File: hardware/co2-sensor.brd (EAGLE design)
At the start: 40 x 44 mm, 21 parts, among them IC1 LM1117IMPX-3.3, J1 MH-Z19, U1 esp12e, U2 dht22, U3 BMP280

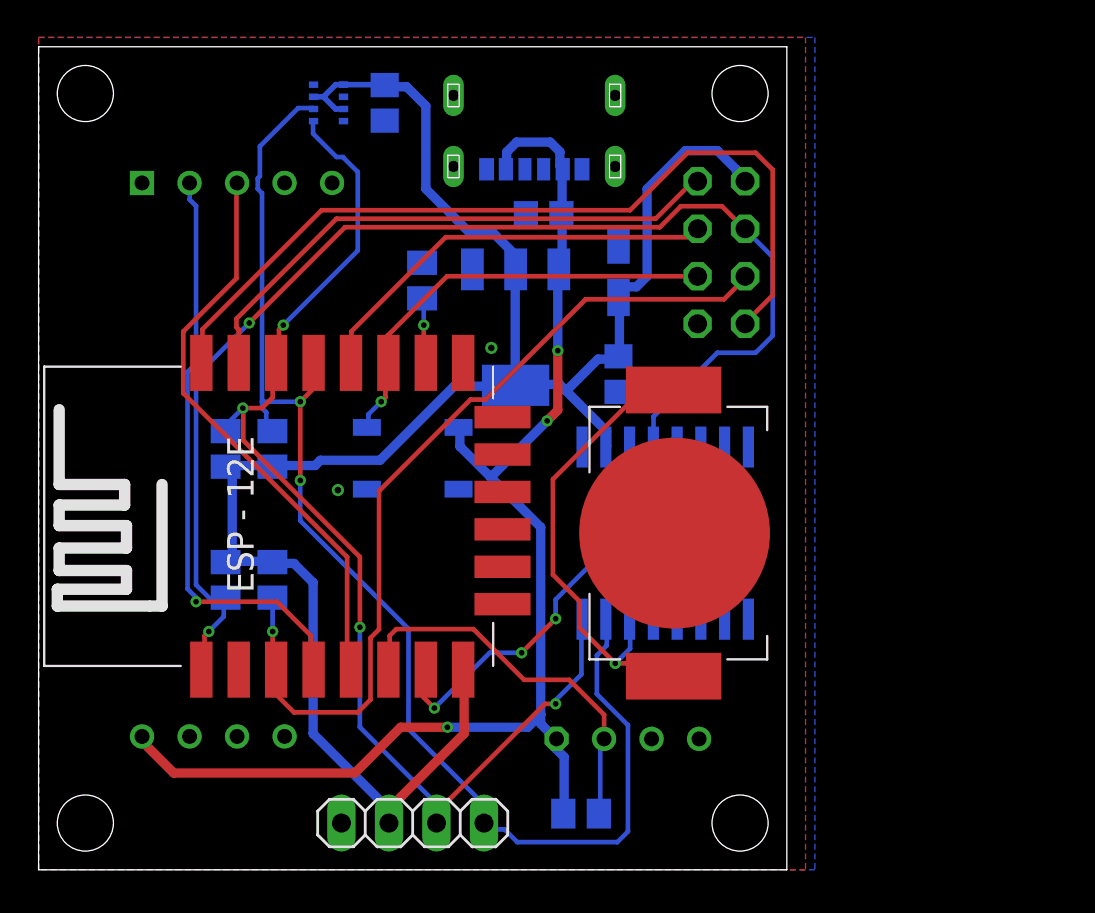
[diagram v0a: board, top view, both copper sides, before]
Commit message: .
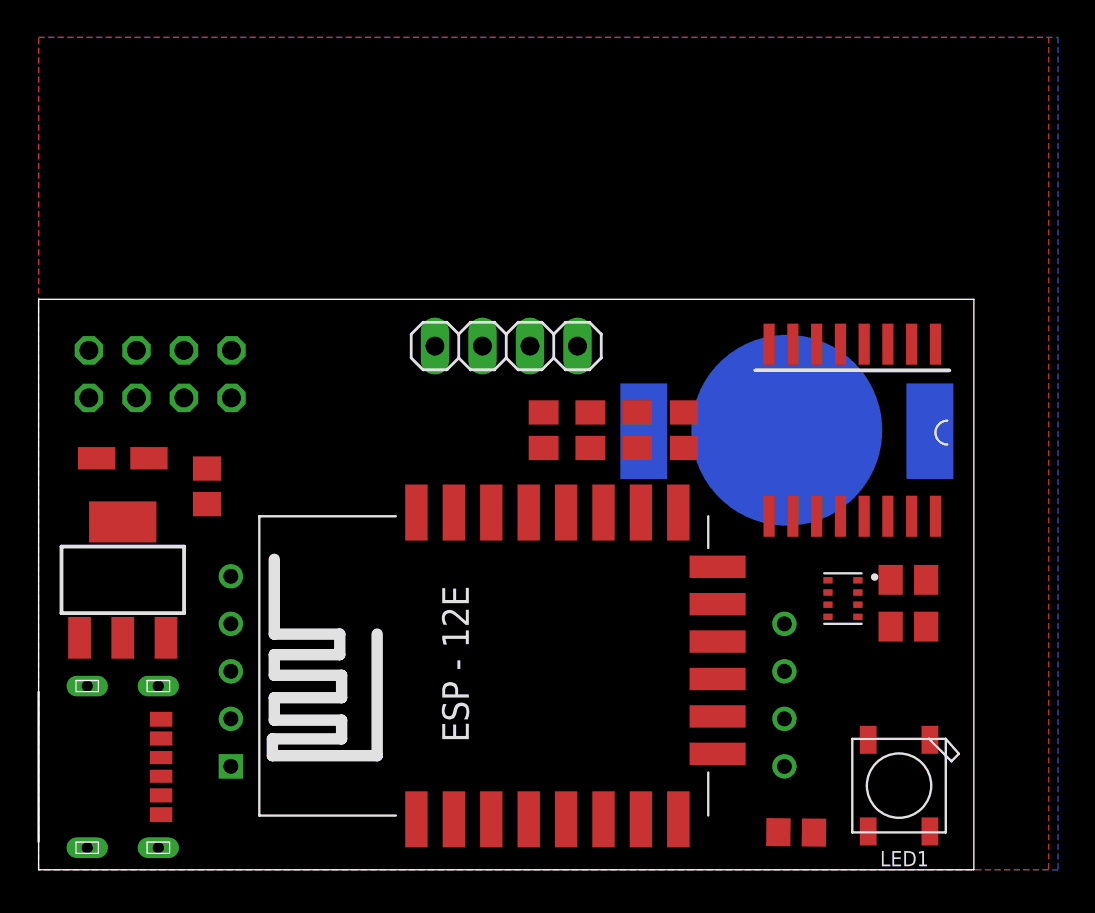
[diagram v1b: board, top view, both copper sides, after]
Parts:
- removed R4: 10k, rcl:M0805
- removed U2: dht22, RHT03_DHT-22_AM2302:AM2302
- moved U$1 46.7 mm to (0.00, 5.50), flipped to the top, turned to 270 degrees
- moved U3 38.2 mm to (43.0, 14.5), flipped to the top
- moved R6 37.7 mm to (46.5, 13.0), flipped to the top, turned to 180 degrees
- moved C4 35.7 mm to (40.5, 2.00), flipped to the top, turned to 179.4 degrees
- moved R5 34.7 mm to (46.5, 15.5), flipped to the top, turned to 180 degrees
- moved J1 33.0 mm to (0.50, 19.5), turned to 0 degrees
- moved LED1 31.3 mm to (46.0, 4.50), flipped to the top, turned to 270 degrees
- moved JP2 30.7 mm to (6.50, 26.5), turned to 0 degrees
- moved C2 28.3 mm to (4.50, 22.0), flipped to the top, turned to 180 degrees
- moved JP1 26.0 mm to (25.0, 28.0)
- moved IC1 25.0 mm to (4.50, 15.5), flipped to the top, turned to 0 degrees
- moved C1 22.6 mm to (9.00, 20.5), flipped to the top
- moved R1 18.8 mm to (29.5, 23.5), flipped to the top
- moved R2 18.8 mm to (27.0, 23.5), flipped to the top
- moved R3 14.0 mm to (32.0, 23.5), flipped to the top
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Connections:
- net +5V: no longer R4.2, U2.VDD
- net DHT22: no longer R4.1, U2.DATA
- net GND: no longer U2.GND
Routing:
- net +3V3: track 105.4 -> 0.00 mm
- net SDA: track 71.0 -> 0.00 mm, vias 2 -> 0
- net +5V: track 69.8 -> 0.00 mm, vias 3 -> 0
- net RST: track 67.2 -> 0.00 mm, vias 2 -> 0
- net SCL: track 62.3 -> 0.00 mm, vias 4 -> 0
- net CH_PD: track 46.7 -> 0.00 mm, vias 1 -> 0
- net TXD: track 45.4 -> 0.00 mm
- net CO2_RX: track 31.7 -> 0.00 mm, vias 1 -> 0
- net CO2_TX: track 30.9 -> 0.00 mm
- net RXD: track 30.1 -> 0.00 mm
- net N$6: track 25.8 -> 0.00 mm, vias 1 -> 0
- net IO2: track 23.3 -> 0.00 mm, vias 1 -> 0
- net IO0: track 22.5 -> 0.00 mm
- net CLOCK_INT: track 21.7 -> 0.00 mm, vias 3 -> 0
- net DHT22: track 20.8 -> 0.00 mm
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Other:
- board size 40 x 44 mm -> 50 x 30.5 mm
